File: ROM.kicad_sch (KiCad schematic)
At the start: 8 parts

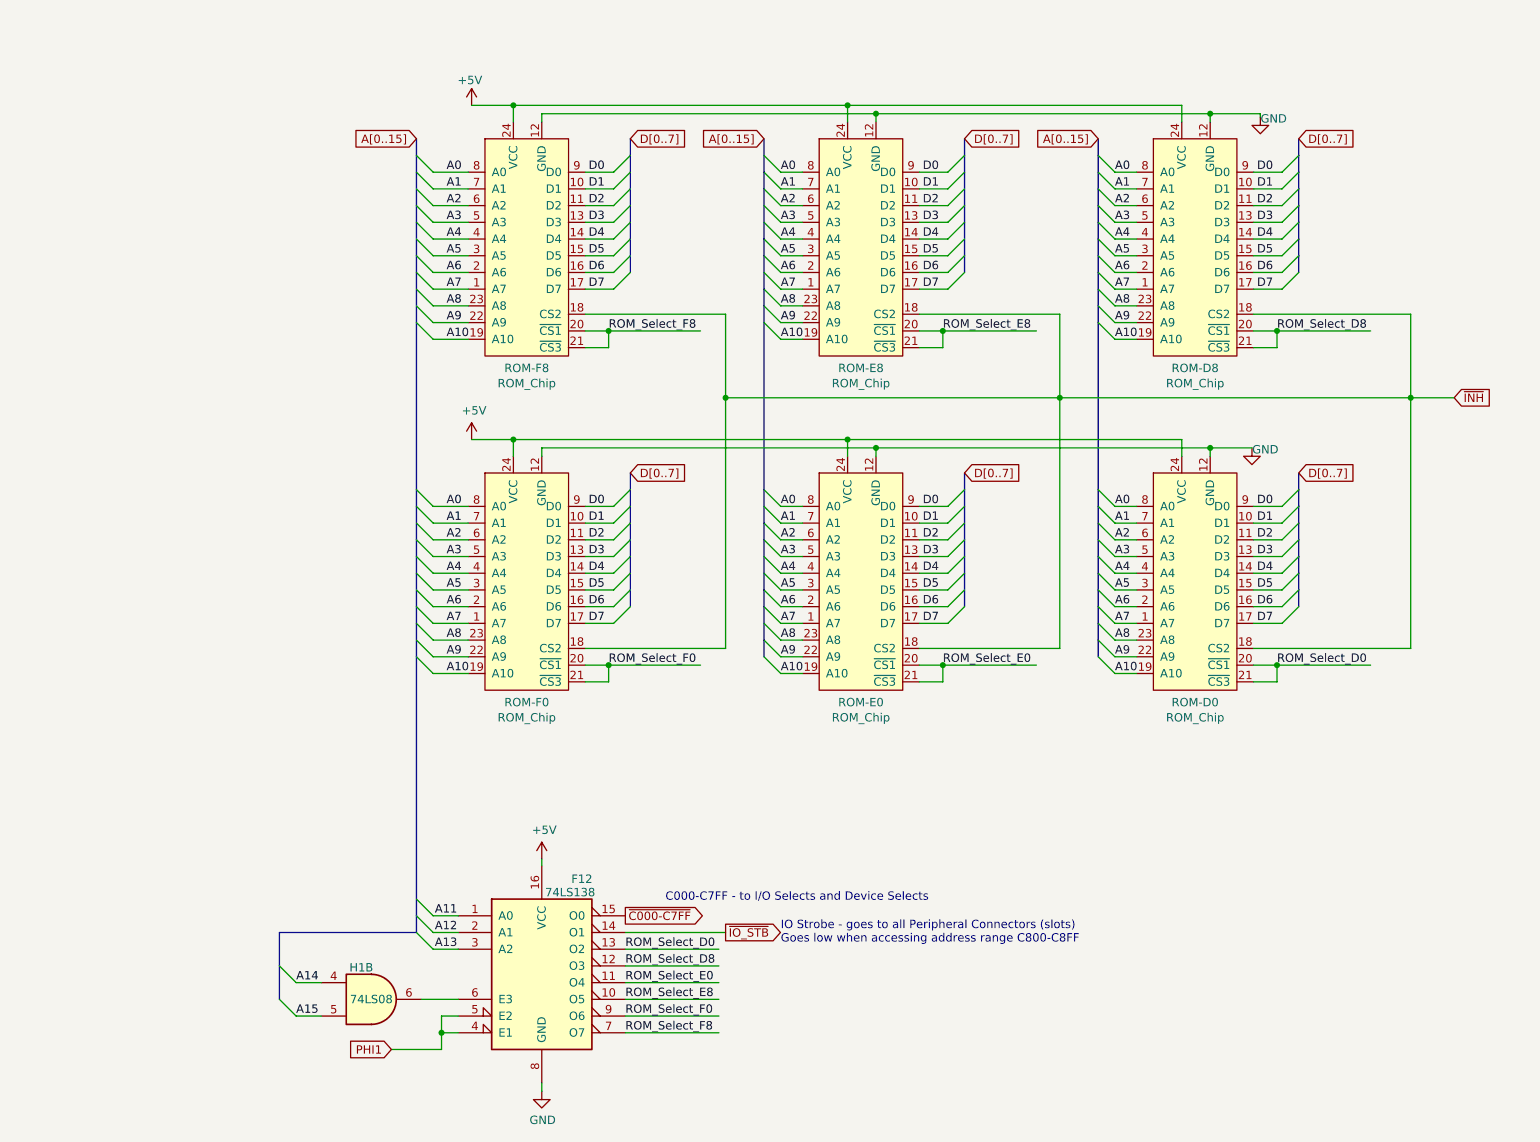
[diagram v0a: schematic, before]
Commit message: Add files via upload
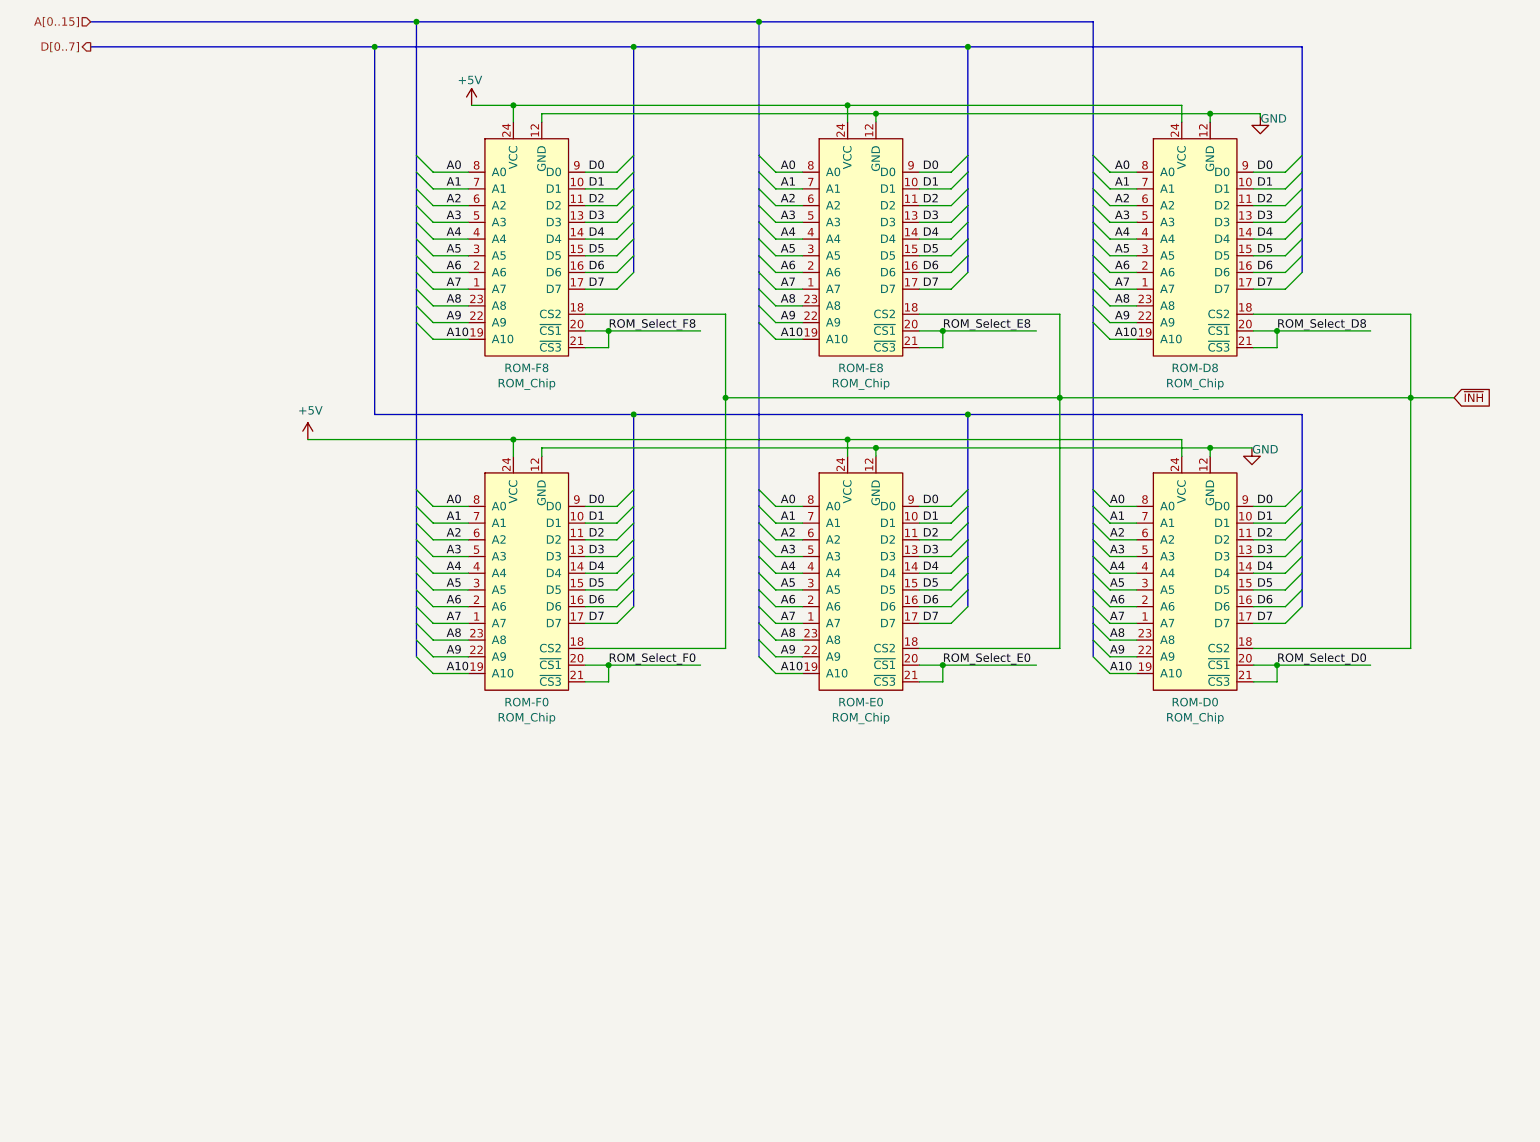
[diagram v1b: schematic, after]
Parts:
- removed F12: 74LS138, Apple:DIP-16_W7.62mm, symbol 74xx:74LS138
- removed H1: 74LS08, Apple:DIP-14_W7.62mm, symbol 74xx:74LS08
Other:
- note removed: "C000-C7FF - to I/O Selects and Device Selects"
- note removed: "IO Strobe - goes to all Peripheral Connectors (slots) Goes low when accessing address range C800-C8FF"
